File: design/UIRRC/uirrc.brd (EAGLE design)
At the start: 51.7 x 83.8 mm, 29 parts, among them IC1 TSOP38438, IC2 MIC5205-3.3YM5-TR, SW1 OMRON_B3SN-3112POMRON_B3SN-31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, SW2 OMRON_B3SN-3112POMRON_B3SN-31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, SW3 OMRON_B3SN-3112POMRON_B3SN-31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, SW4 OMRON_B3SN-3112POMRON_B3SN-31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, SW5 OMRON_B3SN-3112POMRON_B3SN-31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, SW6 OMRON_B3SN-3112POMRON_B3SN-31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, SW7 OMRON_B3SN-3112POMRON_B3SN-31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, SW8 OMRON_B3SN-3112POMRON_B3SN-31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, SW9 OMRON_B3SN-3112POMRON_B3SN-31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, U1 2479, U2 ESP32-WROOM-32E_(16MB)

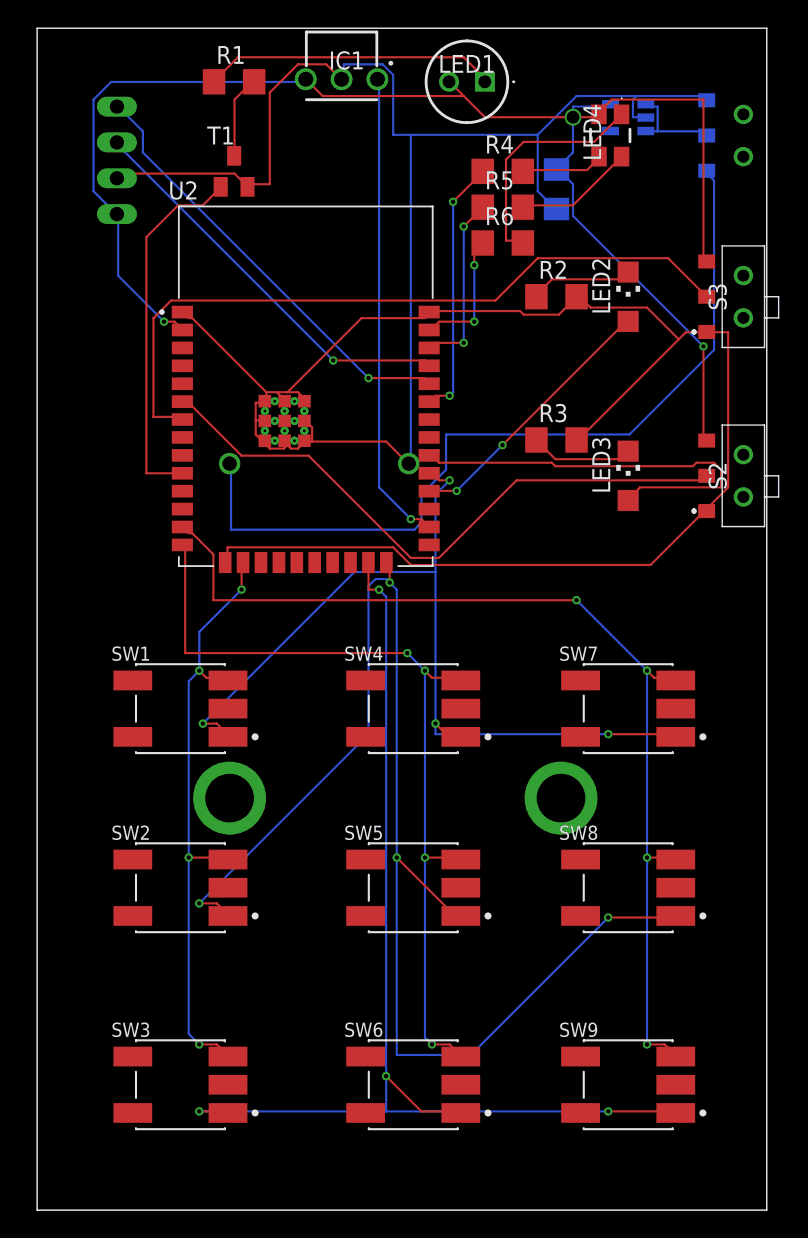
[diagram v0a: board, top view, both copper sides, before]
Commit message: Fixes #12
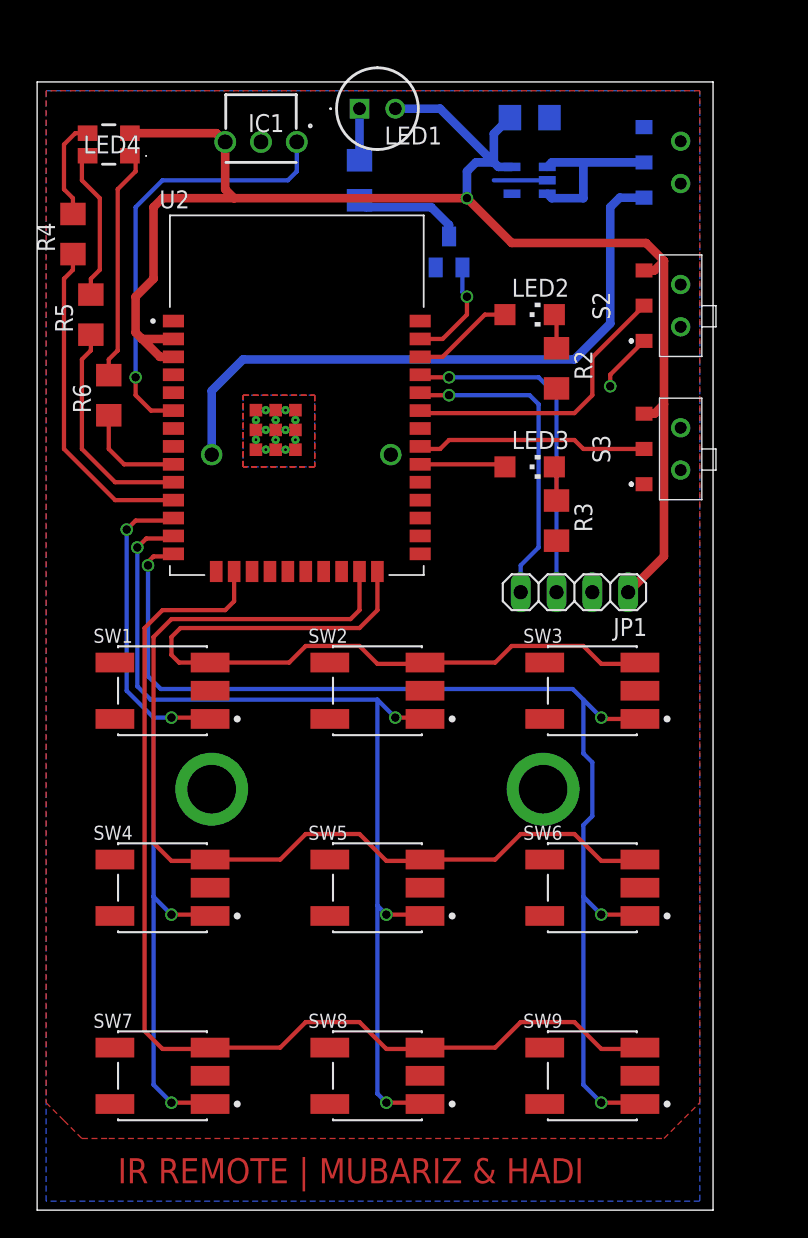
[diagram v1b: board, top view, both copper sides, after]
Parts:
- moved JP1 44.6 mm to (38.1, 43.8), flipped to the top, turned to 180 degrees
- moved SW7 42.0 mm to (8.89, 9.53)
- moved SW3 40.4 mm to (39.4, 36.8)
- moved LED4 35.6 mm to (5.08, 75.6), turned to 180 degrees
- moved R4 30.8 mm to (2.54, 69.2), turned to 90 degrees
- moved R5 30.2 mm to (3.81, 63.5), turned to 90 degrees
- moved R6 30.0 mm to (5.08, 57.8), turned to 90 degrees
- moved SW8 22.2 mm to (24.1, 9.53)
- moved SW4 21.8 mm to (8.89, 22.9)
- moved SW2 19.8 mm to (24.1, 36.8)
- moved SW6 18.9 mm to (39.4, 22.9)
- moved T1 16.3 mm to (29.2, 67.9), flipped to the bottom
- moved S2 12.9 mm to (45.1, 64.1)
- moved S3 11.7 mm to (45.1, 54.0)
- moved R1 11.3 mm to (22.9, 73.0), flipped to the bottom, turned to 270 degrees
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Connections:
- removed net EN: U2.3
- removed net PROFILE_T: U2.31
- net +3V3: now also U2.3
- net BUTTON_C1: now also U2.24; no longer U2.16
- net BUTTON_C2: now also U2.23; no longer U2.14
- net BUTTON_C3: now also U2.16; no longer U2.13
- net BUTTON_R1: now also U2.12; no longer U2.29
- net BUTTON_R2: now also U2.13; no longer U2.24
- net BUTTON_R3: now also U2.14; no longer U2.23
- net IR_RX: now also U2.6; no longer U2.26
- net IR_TX: now also U2.37; no longer U2.10
- net LEARN_EN: now also U2.31; no longer U2.7
- net N$13: now also U2.11; no longer U2.33
- net N$14: now also U2.10; no longer U2.36
- net N$15: now also U2.9; no longer U2.37
- net WIFI_EN: now also U2.33; no longer U2.6
- net WIFI_LED: now also U2.36; no longer U2.28
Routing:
- net GND: track 217.1 -> 8.69 mm, vias 0 -> 1
- net LEARN_EN: track 51.3 -> 16.5 mm
- net BUTTON_R2: track 97.3 -> 69.4 mm
- net LEARN_LED: track 29.6 -> 6.08 mm
- net WIFI_EN: track 44.1 -> 20.7 mm
- net IR_TX: track 26.1 -> 7.51 mm, vias 0 -> 1
- net N$1: track 20.8 -> 3.66 mm
- net N$11: track 59.8 -> 45.7 mm
- net WIFI_LED: track 19.1 -> 7.25 mm, vias 2 -> 0
- net BUTTON_C1: track 43.8 -> 55.0 mm, vias 4 -> 0
- net BUTTON_C2: track 60.0 -> 71.0 mm, vias 4 -> 0
- net USB_TXD: track 31.2 -> 22.6 mm
- net BUTTON_R1: track 62.7 -> 57.0 mm
- net N$16: track 7.27 -> 12.2 mm
- net N$13: track 18.5 -> 23.3 mm, vias 2 -> 0
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- added copper zone on layer 1, net GND
- added copper zone on layer 16, net GND
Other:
- board size 51.7 x 83.8 mm -> 47.9 x 80 mm
- board text added: "IR REMOTE | MUBARIZ & HADI"
